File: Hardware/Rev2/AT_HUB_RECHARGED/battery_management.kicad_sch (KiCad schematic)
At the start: 39 parts, among them J13 Pack Thermister, J14 Through Hole, J15 EXT Charge Port, J16 USB_C_Receptacle_PowerOnly_6P, J2 JST, Q1 NTR1P02T1G, Q2 NTR1P02T1G, SW11 SW_SPDT, U7 BQ21040DBV, U8 TLV61070ADBV, U9 BQ27427YZFR

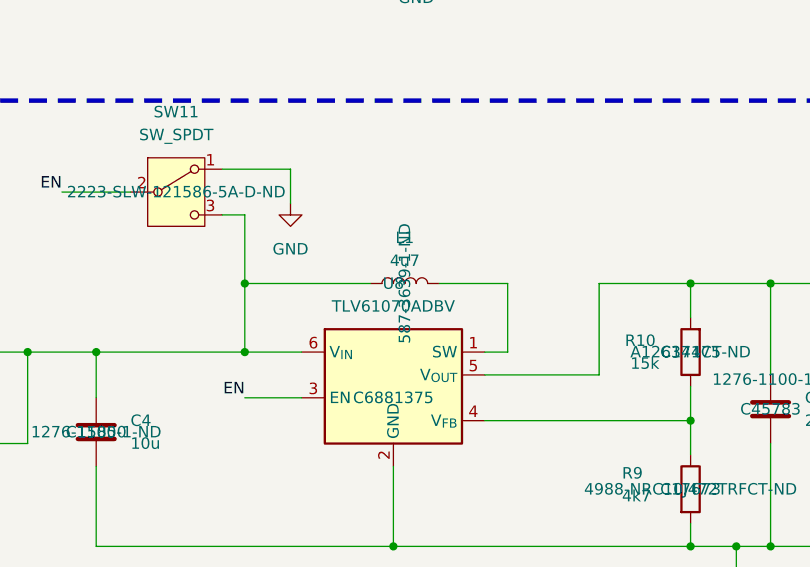
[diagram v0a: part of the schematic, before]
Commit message: A
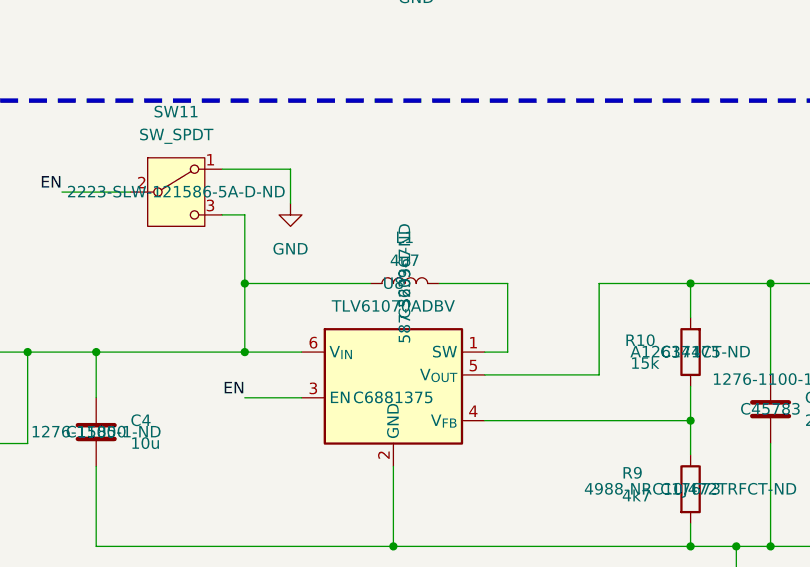
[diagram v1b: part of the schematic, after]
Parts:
- L1: LCSC (none) -> C520367
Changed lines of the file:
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@@
 			)
 		)
-		(property "LCSC" ""
+		(property "LCSC" "C520367"
 			(at 189.23 125.73 0)
 			(effects
